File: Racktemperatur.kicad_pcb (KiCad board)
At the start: 2 copper layers, 67.6 x 57.5 mm, 20 parts, among them J1 Conn_01x03, J2 Conn_01x03, J3 Barrel_Jack_MountingPin, Q1 IRLZ44N, U1 74HC595, U2 74HC595, U3 DS18B20

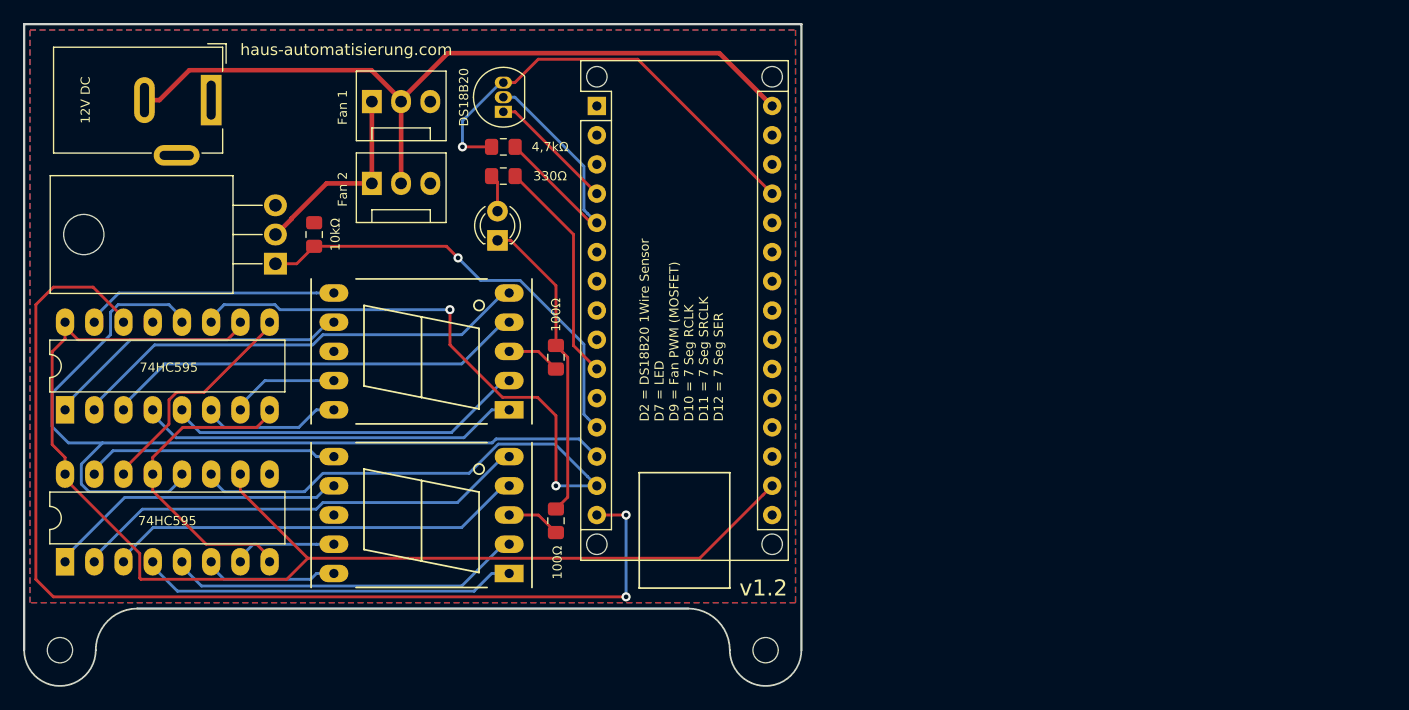
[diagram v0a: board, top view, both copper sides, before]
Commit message: Version 1.3 as rack mount
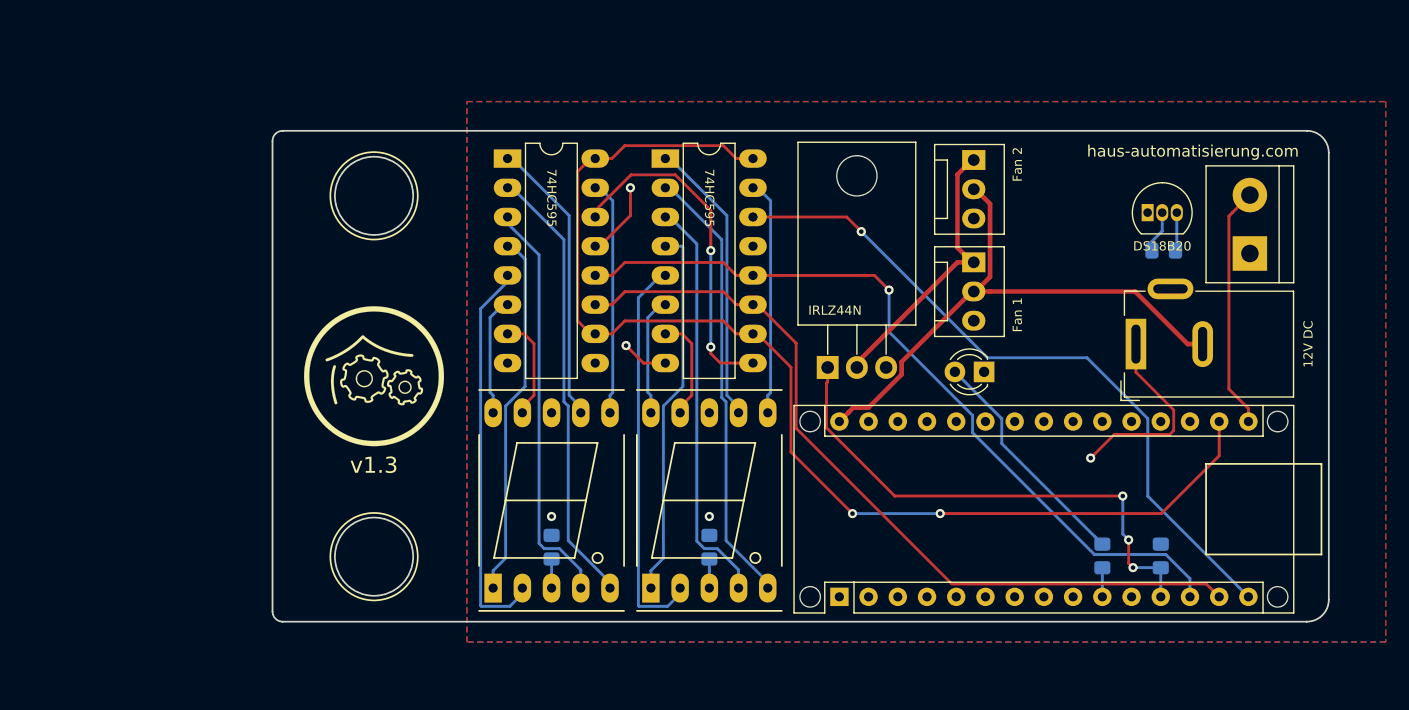
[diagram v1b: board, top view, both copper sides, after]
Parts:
- removed the REF** at (145.7, 125.5)
- removed the REF** at (84.4, 125.5)
- added G***: LOGO, libs:Logo, F.Cu at (111.7, 101.7)
- added J4: Screw_Terminal_01x02, TerminalBlock:TerminalBlock_bornier-2_P5.08mm, F.Cu at (187.8, 91.1)
- R1, R2, R3, R4, R5: moved to B.Cu
- moved J3 83.1 mm to (177.9, 98.9), turned to 90 degrees
- moved R4 78.7 mm to (180.1, 117.3)
- moved REF** 65.0 mm to (190.0, 115.4)
- moved R5 61.7 mm to (175.0, 117.3), turned to 90 degrees
- moved R3 58.1 mm to (180.3, 90.8), turned to 180 degrees
- moved U3 56.7 mm to (178.9, 87.5), turned to 0 degrees
- moved U1 56.6 mm to (137.0, 82.8), turned to 0 degrees
- moved J2 52.8 mm to (163.8, 91.8), turned to 270 degrees
- moved J1 52.6 mm to (163.8, 82.9), turned to 270 degrees
- moved U2 52.0 mm to (123.3, 82.8), turned to 0 degrees
- moved Q1 48.8 mm to (151.1, 101.0), turned to 0 degrees
- moved A1 47.6 mm to (152.1, 120.9), turned to 90 degrees
- moved D1 43.8 mm to (164.7, 101.3), turned to 180 degrees
- moved R1 21.2 mm to (140.8, 116.6)
- moved G*** 20.7 mm to (111.7, 101.7), turned to 180 degrees
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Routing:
- net GND: track 66.4 -> 27.7 mm, vias 0 -> 5
- net Net-(A1-Pad27): track 38.8 -> 3.35 mm, vias 1 -> 0
- net Net-(A1-Pad15): track 95.2 -> 60.7 mm, vias 2 -> 1
- net Net-(A1-Pad16): track 0.00 -> 21.1 mm
- net Net-(A1-Pad5): track 24.7 -> 3.67 mm
- net +12V: track 67.6 -> 49.0 mm
- net Net-(A1-Pad10): track 19.7 -> 2.53 mm
- net Net-(D1-Pad2): track 3.26 -> 20.3 mm
- net Net-(A1-Pad13): track 82.3 -> 68.1 mm, vias 0 -> 1
- net Net-(A1-Pad14): track 83.9 -> 70.0 mm, vias 2 -> 0
- net Net-(U1-Pad9): track 19.9 -> 29.6 mm, vias 0 -> 2
- net Net-(A1-Pad17): track 111.4 -> 102.6 mm, vias 0 -> 2
- net Net-(J1-Pad1): track 17.4 -> 24.4 mm
- net Net-(A1-Pad12): track 38.7 -> 45.0 mm, vias 1 -> 3
- net Net-(AFF2-Pad2): track 31.1 -> 34.3 mm
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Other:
- board size 67.6 x 57.5 mm -> 91.8 x 42.7 mm
- board text added: "D2 = DS18B20 1Wire Sensor D7 = LED D9 = Fan PWM (MOSFET) D10 = 7 Seg RCLK D11 = 7 Seg SRCLK D12 = 7 Seg SER D13 = Terminal"
- board text added: "IRLZ44N"
- board text added: "v1.3"
- board text removed: "D2 = DS18B20 1Wire Sensor D7 = LED D9 = Fan PWM (MOSFET) D10 = 7 Seg RCLK D11 = 7 Seg SRCLK D12 = 7 Seg SER"
- board text removed: "v1.2"
